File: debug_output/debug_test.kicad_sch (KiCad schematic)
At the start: 1 part

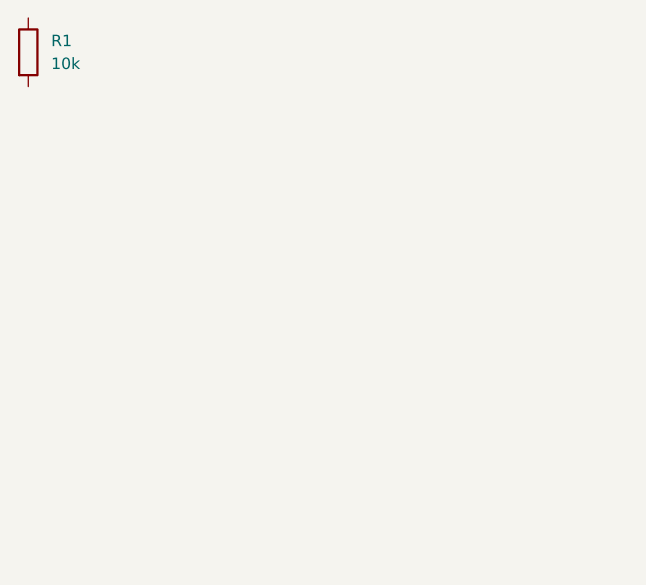
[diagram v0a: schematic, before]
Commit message: continue to troubleshooting
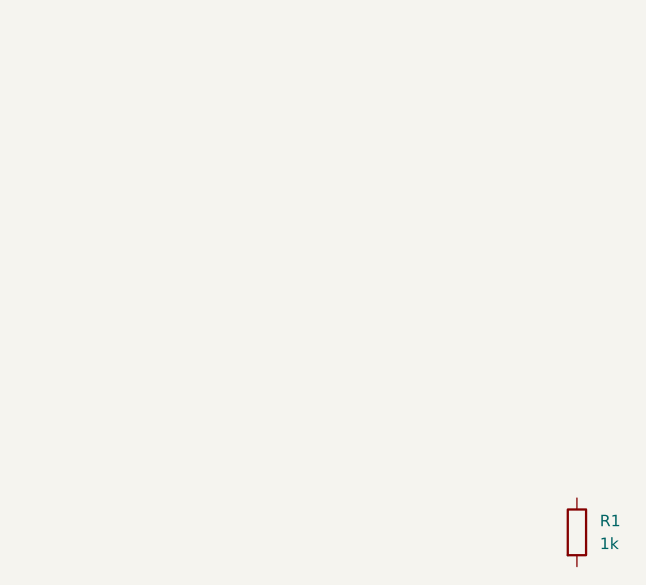
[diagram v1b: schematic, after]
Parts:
- R1: value 10k -> 1k; footprint Resistor_SMD:R_0805_2012Metric -> Resistor_SMD:R_0603_1608Metric
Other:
- title: top -> test_circuit
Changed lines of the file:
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@@
 	(version 20250114)
 	(generator "kicad_api")
-	(generator_version 9.0)
-	(paper A4)
-	(paper A4)
+	(generator_version "9.0")
+	(paper "A4")
 	(title_block
-		(title top)
+		(title test_circuit)
 		(date 2025-08-04)
 		(company Circuit-Synth)
 	)
 	(symbol
-		(lib_id Device:R)
-		(at 38.1 45.72 0)
+		(lib_id "Device:R")
+		(at 99.06 99.06 0)
 		(in_bom yes)
 		(on_board yes)
 		(dnp no)
-		(property
-			"Reference"
-			"R1"
-			(at 40.64 44.449999999999996 0)
+		(property "Reference" "R1"
+			(at 101.60000000000001 97.79 0)
 			(effects
 				(font
@@
 			)
 		)
-		(property
-			"Value"
-			"10k"
-			(at 40.64 46.99 0)
+		(property "Value" "1k"
+			(at 101.60000000000001 100.33 0)
 			(effects
 				(font
@@
 			)
 		)
-		(property
-			"Footprint"
-			"Resistor_SMD:R_0805_2012Metric"
-			(at 38.1 55.72 0)
+		(property "Footprint" "Resistor_SMD:R_0603_1608Metric"
+			(at 99.06 109.06 0)
 			(effects
 				(font
@@
 		(instances
 			(project
-				"circuit"
+				"debug_test"
 				(path
 					"/"
-					(reference R1)
-					(unit 1)
-				)
-			)
-			(project
-				"generated_project"
-				(path
-					"/50b29d65-f667-46a0-bc9a-63b22f4f45f1"
-					(reference R1)
+					(reference "R1")
 					(unit 1)
 				)
@@
 	(sheet_instances
 		(path
-			"/50b29d65-f667-46a0-bc9a-63b22f4f45f1"
+			"/"
 			(page "1")
 		)
 	)
 	(embedded_fonts no)
-	(sheet_instances
-		(path
-			"/"
-			(page "1")
-		)
-	)
 )
